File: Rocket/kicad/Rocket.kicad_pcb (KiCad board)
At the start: 2 copper layers, 133.6 x 110.8 mm, 23 parts, among them Q1 Q_NPN_EBC, Q2 Q_NPN_EBC, U1 NE555P, U2 BAT_HLD_SMD

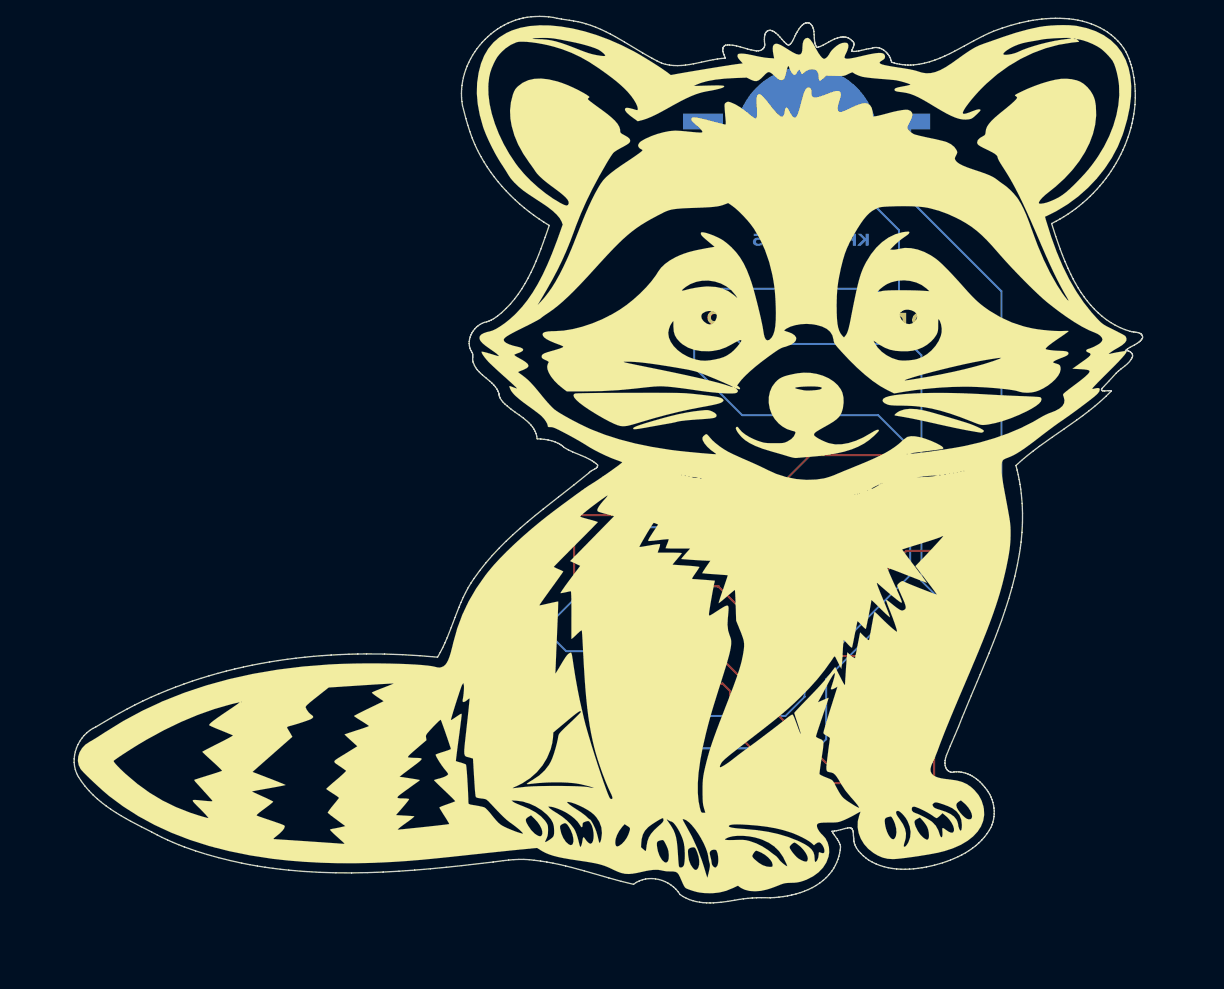
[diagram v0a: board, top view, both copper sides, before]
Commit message: V08122025
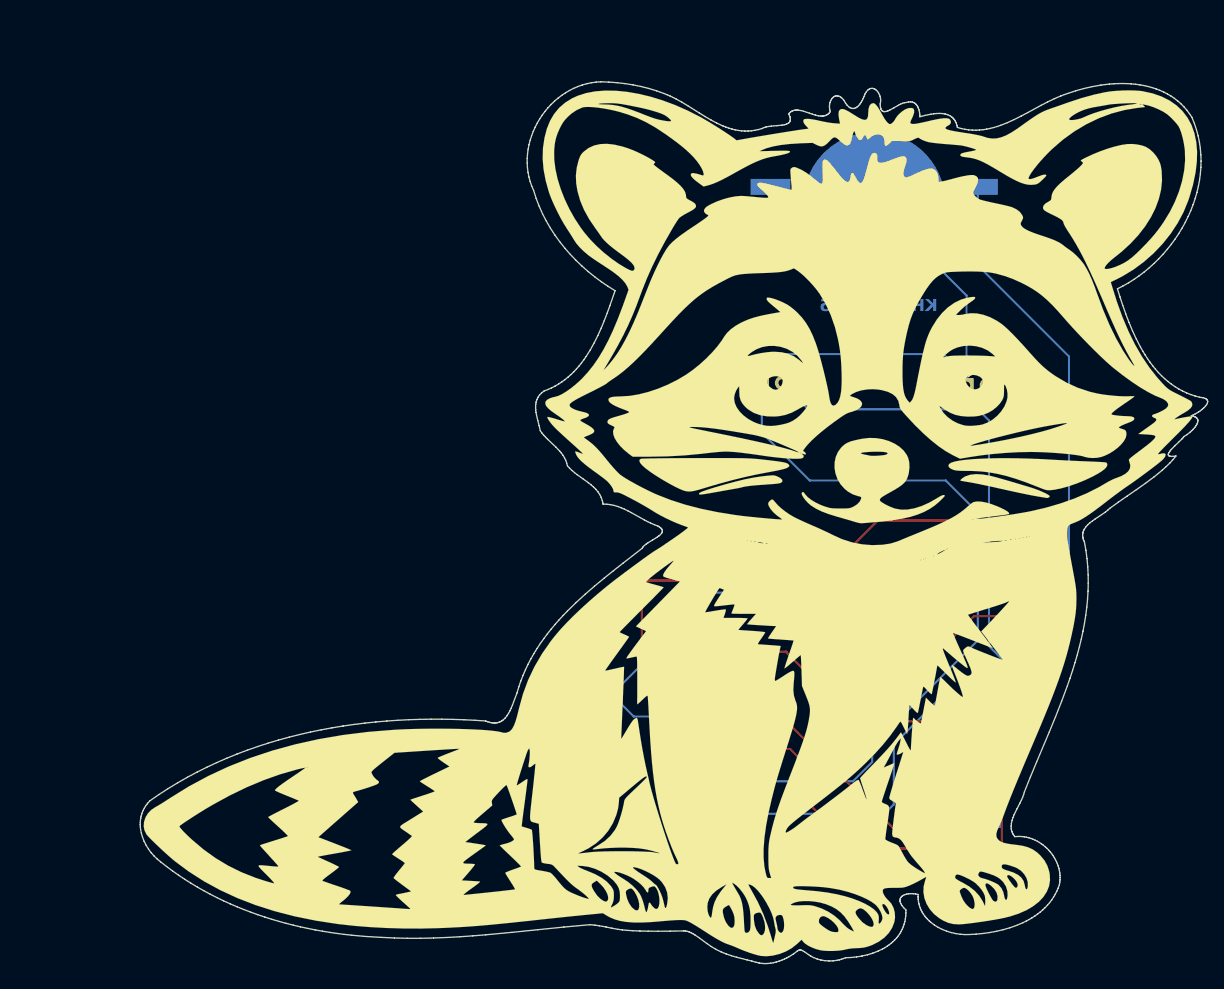
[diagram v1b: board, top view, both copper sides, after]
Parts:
- removed the G*** at (136.8, 95.3) (x7)
- added G*** (x6): LOGO, LOGO, F.Cu at (145.2, 103.4)
- added G*** (x7): LOGO, LOGO, F.Cu at (145.0, 103.4)
- moved C1 11.7 mm to (158.2, 120.8)
- moved D1 11.7 mm to (172.5, 78.8)
- moved D2 11.7 mm to (146.9, 78.5)
- moved D3 11.7 mm to (156.3, 100.9)
- moved G*** 11.7 mm to (166.9, 92.2)
- moved Q1 11.7 mm to (172.8, 120.5)
- moved R3 11.7 mm to (135.8, 132.3)
- moved R4 11.7 mm to (135.8, 128.3)
- moved R5 11.7 mm to (135.8, 124.2)
- moved R6 11.7 mm to (135.8, 120.2)
- moved S1 11.7 mm to (181.2, 110.2)
- moved U1 11.7 mm to (156.3, 112.3)
- moved U2 11.7 mm to (161.0, 56.0)
- moved Q2 11.7 mm to (169.5, 130.6)
- moved R7 11.7 mm to (135.8, 116.1)
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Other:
- board size 133.6 x 110.8 mm -> 133.4 x 110.2 mm

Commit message: V10122025
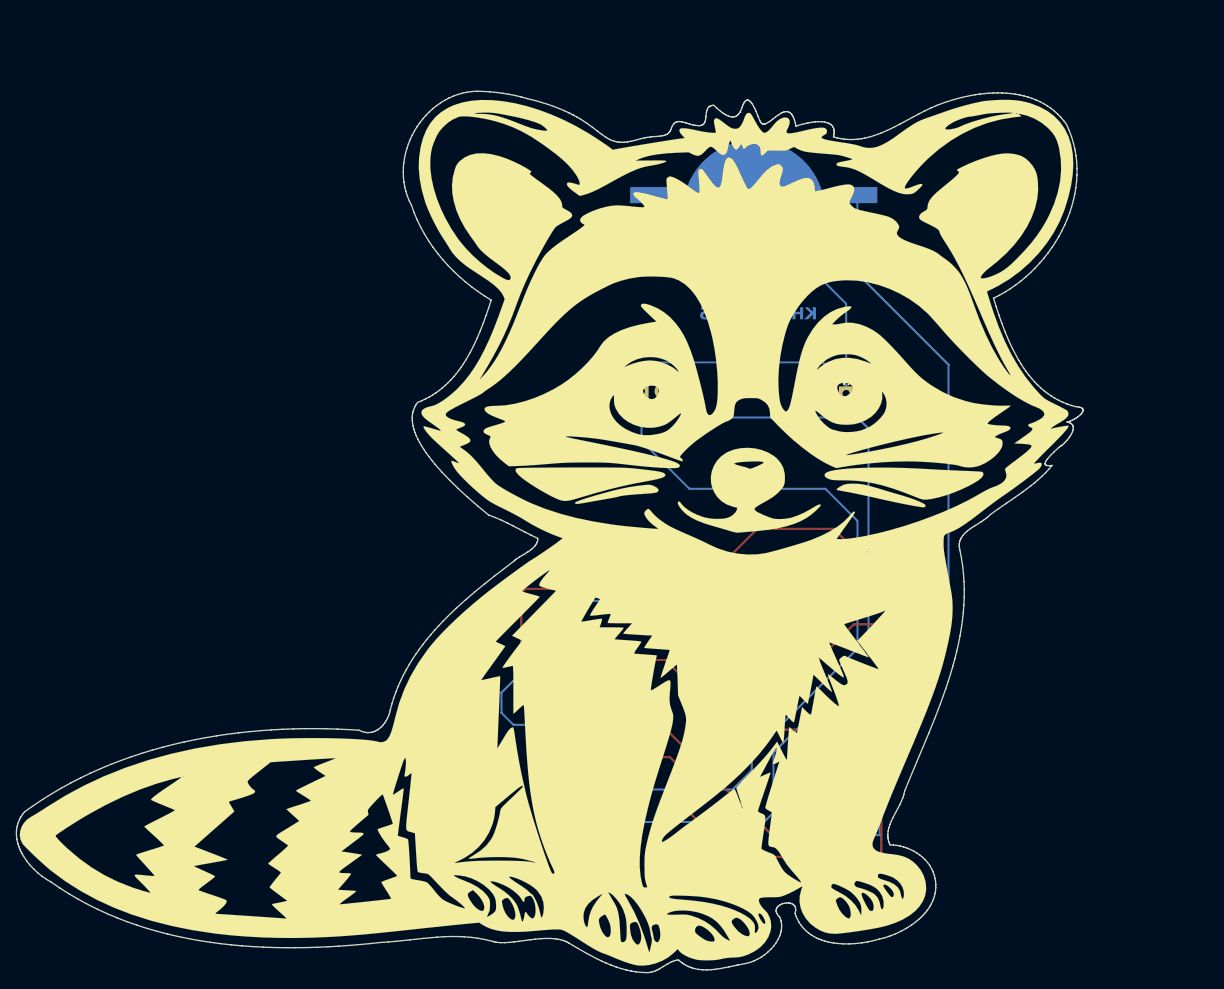
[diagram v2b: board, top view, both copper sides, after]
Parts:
- removed the G*** at (145.2, 103.4) (x6)
- removed the G*** at (145.0, 103.4) (x7)
- added G*** (x7): LOGO, LOGO, F.Cu at (129.5, 104.6)
- added G*** (x6): LOGO, LOGO, F.Cu at (130.2, 104.5)
- added G*** (x6): LOGO, LOGO, F.Cu at (130.0, 104.5)
- moved C1 15.1 mm to (143.2, 121.8)
- moved D3 15.1 mm to (141.2, 101.9)
- moved S1 15.1 mm to (166.2, 111.2)
- moved R4 15.1 mm to (120.7, 129.3)
- moved R7 15.1 mm to (120.7, 117.2)
- moved R3 15.1 mm to (120.7, 133.3)
- moved R5 15.1 mm to (120.7, 125.2)
- moved R6 15.1 mm to (120.7, 121.2)
- moved R8 15.1 mm to (120.7, 113.1)
- moved Q2 15.1 mm to (154.5, 131.6)
- moved D1 15.1 mm to (157.5, 79.8)
- moved D2 15.1 mm to (131.9, 79.5)
- moved G*** 15.1 mm to (151.9, 93.2)
- moved Q1 15.1 mm to (157.7, 121.5)
- moved U1 15.1 mm to (141.2, 113.3)
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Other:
- board size 133.4 x 110.2 mm -> 133.3 x 110.2 mm
